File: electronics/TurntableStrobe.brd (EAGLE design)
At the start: 25.1 x 17.8 mm, 16 parts, among them IC1 TINY25, J1 ISP, Q1 12MHz

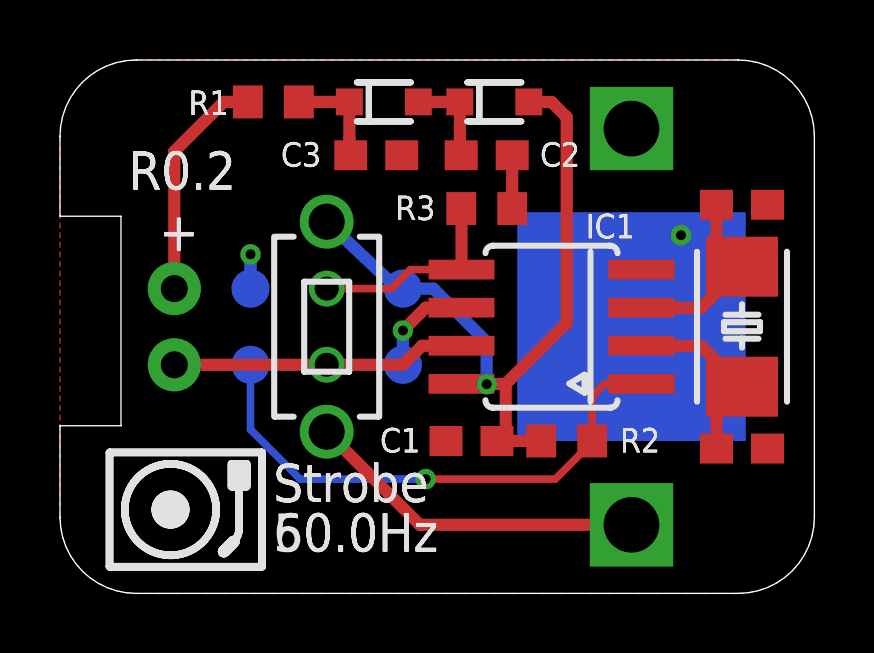
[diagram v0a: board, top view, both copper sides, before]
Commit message: added solder jumper for easier reprogramming. Minor silk tweaks. New logo.
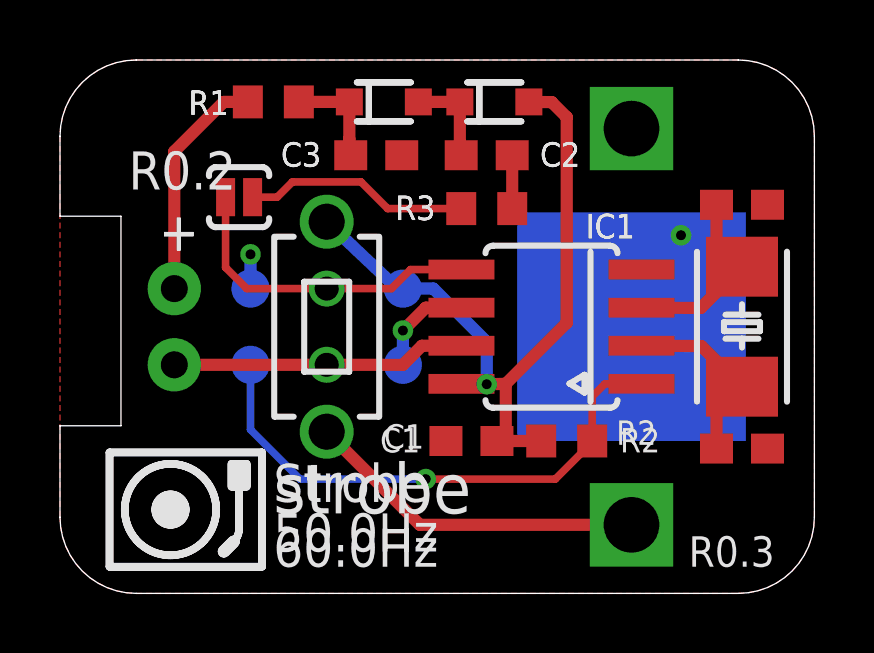
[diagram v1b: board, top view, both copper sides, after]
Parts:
- added JP1: pgm, SparkFun-Retired:SJ_2S-NO
- added U$5: BTLOGO-LOGO-MD, bt:BTLOGOM
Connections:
- new net N$1: JP1.2, R3.2
- net PB0: now also JP1.1; no longer R3.2
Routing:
- net N$1: track 0.00 -> 7.53 mm
- net PB0: track 6.79 -> 10.8 mm
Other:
- board text added: "R0.3"
- board text added: "cc-by-sa"
- board text added: "strobe"
